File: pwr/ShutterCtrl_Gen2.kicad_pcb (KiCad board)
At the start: 2 copper layers, 94 x 94 mm, 17 parts, among them K1 G2RL-2, Q1 BC817, Q2 TSM500P02CX, U1 S216S02

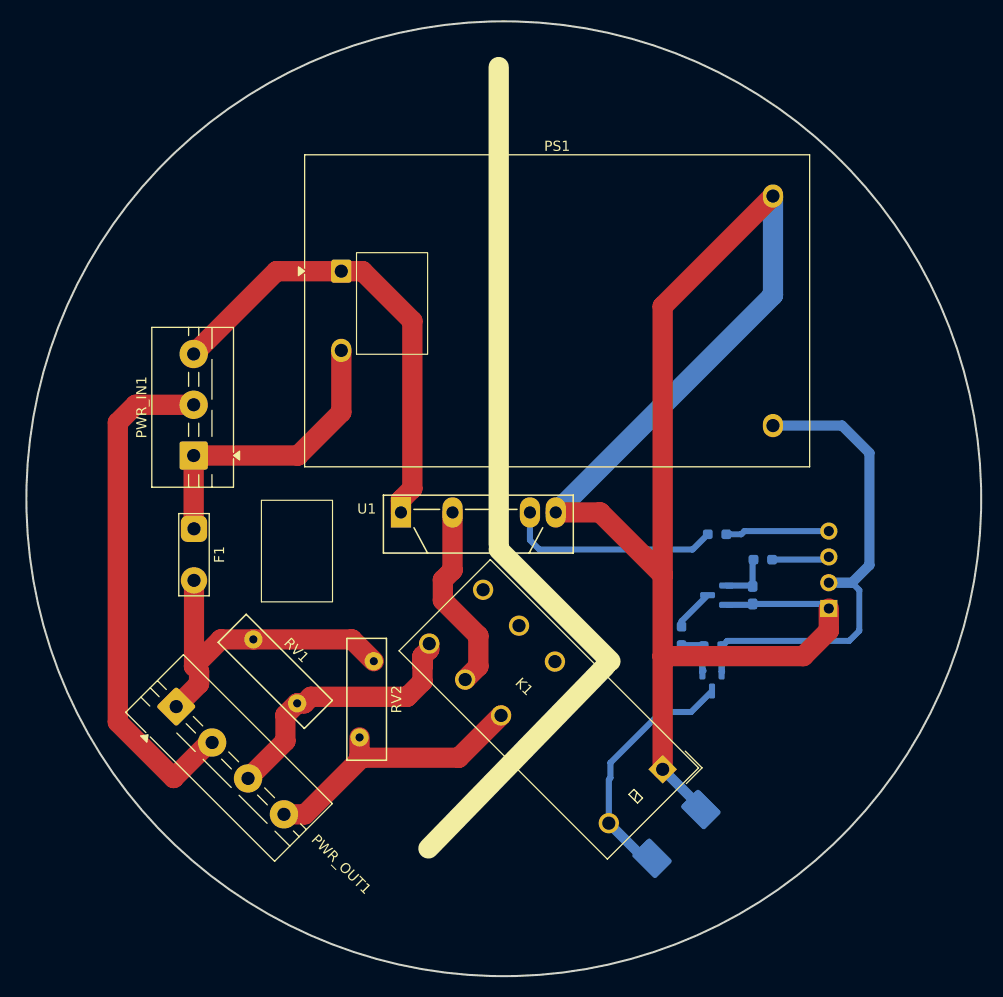
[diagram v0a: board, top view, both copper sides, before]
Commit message: First version of HW design
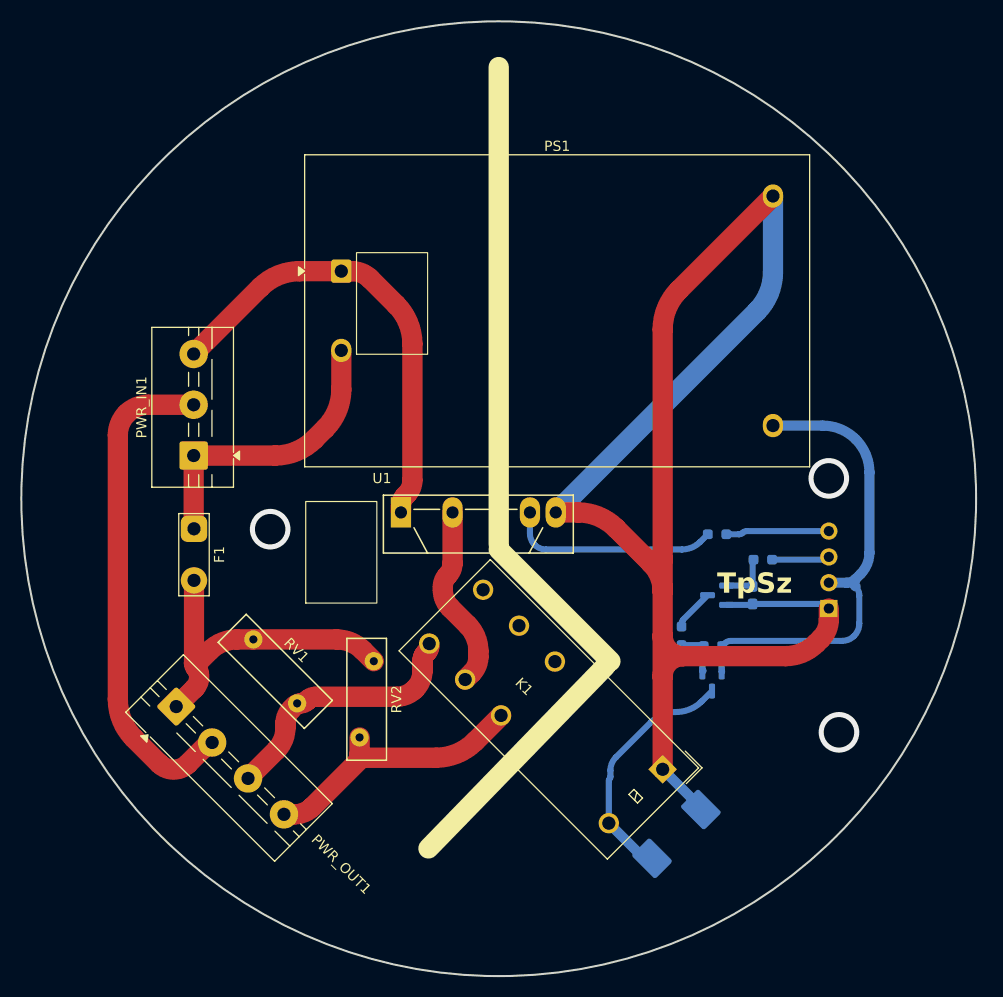
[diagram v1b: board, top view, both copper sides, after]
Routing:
- net GND: track 149.4 -> 155.3 mm
- net PE: track 50.7 -> 49.2 mm
- net L: track 46.3 -> 45.4 mm
- net L_RELAY: track 18.8 -> 18.3 mm
- net N: track 29.6 -> 29.1 mm
- net (no net): vias 0 -> 3
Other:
- board text added: "TpSz"
